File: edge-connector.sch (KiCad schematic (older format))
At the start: 3 parts

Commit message: Fixed libs
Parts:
- J?: footprint _autosave-artix-dc-scm-footprints:SFF-TA-1002-4C+ -> artix-dc-scm-footprints:SFF-TA-1002-4C+; symbol _autosave-artix-dc-scm:SFF-TA-1002-4C+ -> artix-dc-scm:SFF-TA-1002-4C+
- R136, R137: footprint _autosave-artix-dc-scm-footprints:0402-res -> artix-dc-scm-footprints:0402-res; symbol _autosave-artix-dc-scm:R_0R_0402 -> artix-dc-scm:R_0R_0402
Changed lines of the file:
@@
 Connection ~ 6925 10425
 $Comp
-L _autosave-artix-dc-scm:GND-artix-dc-scm #PWR026
+L artix-dc-scm:GND-artix-dc-scm #PWR026
 U 1 1 626F241B
 P 6925 10625
@@
 	8825 10425 8825 10625
 $Comp
-L _autosave-artix-dc-scm:GND-artix-dc-scm #PWR027
+L artix-dc-scm:GND-artix-dc-scm #PWR027
 U 1 1 62BB82B7
 P 8825 10625
@@
 $EndComp
 $Comp
-L _autosave-artix-dc-scm:R_0R_0402 R136
+L artix-dc-scm:R_0R_0402 R136
 U 1 1 616ABCDE
 P 9050 6725
 F 0 "R136" H 9050 6938 60  0000 C CNN
 F 1 "R_0R_0402" H 9050 6575 60  0001 C CNN
-F 2 "_autosave-artix-dc-scm-footprints:0402-res" H 9250 6925 60  0001 L CNN
+F 2 "artix-dc-scm-footprints:0402-res" H 9250 6925 60  0001 L CNN
 F 3 "" H 9050 6725 50  0001 C CNN
 F 4 "PANASONIC" H 9250 7125 60  0001 L CNN "Manufacturer"
@@
 SGPIO0_CLK
 $Comp
-L _autosave-artix-dc-scm:R_0R_0402 R137
+L artix-dc-scm:R_0R_0402 R137
 U 1 1 617019A6
 P 10275 6725
 F 0 "R137" H 10275 6938 60  0000 C CNN
 F 1 "R_0R_0402" H 10275 6575 60  0001 C CNN
-F 2 "_autosave-artix-dc-scm-footprints:0402-res" H 10475 6925 60  0001 L CNN
+F 2 "artix-dc-scm-footprints:0402-res" H 10475 6925 60  0001 L CNN
 F 3 "" H 10275 6725 50  0001 C CNN
 F 4 "PANASONIC" H 10475 7125 60  0001 L CNN "Manufacturer"
@@
 PCIE_HPM_TX[0]_P
 $Comp
-L _autosave-artix-dc-scm:SFF-TA-1002-4C+ J?
+L artix-dc-scm:SFF-TA-1002-4C+ J?
 U 1 1 601205AF
 P 7875 1425
 F 0 "J?" H 7875 1590 50  0000 C CNN
 F 1 "SFF-TA-1002-4C+" H 7875 1499 50  0000 C CNN
-F 2 "_autosave-artix-dc-scm-footprints:SFF-TA-1002-4C+" H 8025 1475 50  0001 C CNN
+F 2 "artix-dc-scm-footprints:SFF-TA-1002-4C+" H 8025 1475 50  0001 C CNN
 F 3 "https://cdn.amphenol-icc.com/media/wysiwyg/files/documentation/sme005.pdf?__cf_chl_jschl_tk__=4604d1306574a1ee474ea914090d3e0c57e266a6-1606907014-0-AbkYBTCTl__kMBcY3BDmgKpfUy32FqitwN2Lniuy8W-uyv2Ev04Q-Q5Mr7srIz_Wnur0_9chB4CRbxKSYcEh7IvAJYsUgJ0PWIS5YdRqqHg567uaZciEX2hQP4ss5l6M4XdNrxEjJppHvyRV3ku89t-VmUSzhgCb8oJlyHpTxST4dEmKZNXfM53TM0tmGirdVbCRt1Byrx5pkz_uMvNABIOj7B2-eDGK52J3DWRD76zEyjdxY7Iz11gPiOY5i_QGIR3uOwkR5LBPNXe8zGqAf8--AKa7RqDbIriQRt90_32C4zIuHqbGa05BXS135E65ov80PbVcb4eSiutCqcJUAacUwu3eVnXVeIumfihJxuP8Rv7_n6saeG_2IuQpEiskzovLGKZM3667Y-rm-AL1NRXTamtvBxqTk0vyMvZ60FgJ" H 8075 1375 50  0001 C CNN
 	1    7875 1425

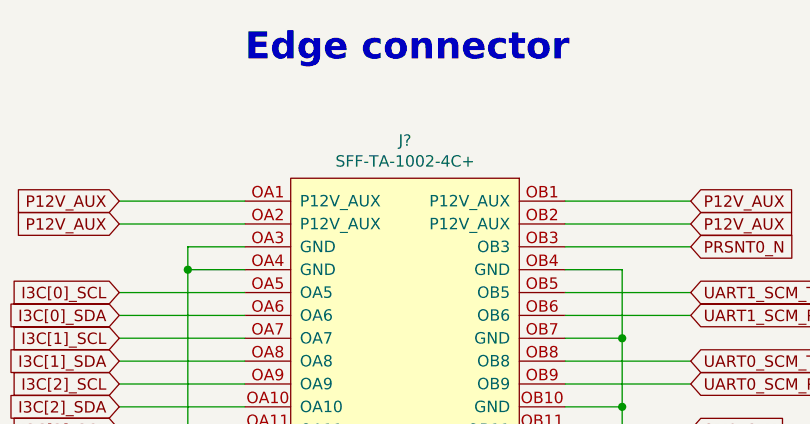
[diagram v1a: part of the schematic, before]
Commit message: update loclib
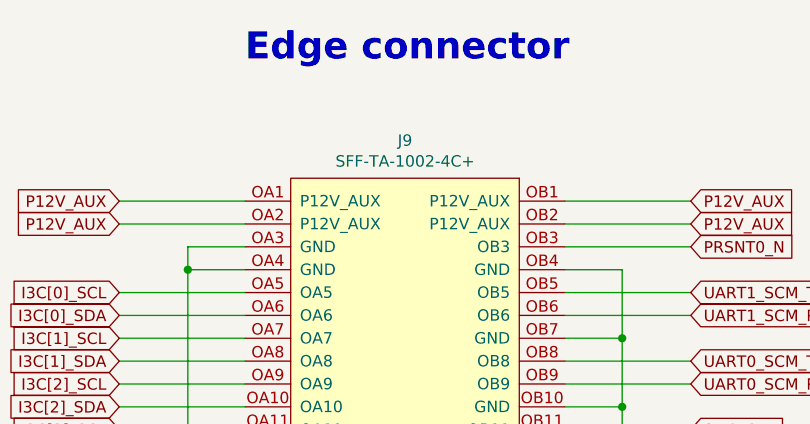
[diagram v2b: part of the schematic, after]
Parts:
- removed J?: SFF-TA-1002-4C+, artix-dc-scm-footprints:SFF-TA-1002-4C+, symbol artix-dc-scm:SFF-TA-1002-4C+
- added J9: SFF-TA-1002-4C+, artix-dc-scm-footprints:SFF-TA-1002-4C+, symbol artix-dc-scm:SFF-TA-1002-4C+
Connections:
- net 3V0_BAT: now also J9.B41
- net CHASI#: now also J9.A54
- net DBP_PRDY_N: now also J9.A50
- net DBP_PREQ_N: now also J9.A49
- net ESPI_ALERT_N: now also J9.B3
- net ESPI_CLK: now also J9.B1
- net ESPI_CS0_N: now also J9.B2
- net ESPI_CS1_N: now also J9.B9
- net ESPI_IO0: now also J9.B5
- net ESPI_IO1: now also J9.B6
- net ESPI_IO2: now also J9.B7
- net ESPI_IO3: now also J9.B8
- net ESPI_RESET_N: now also J9.B4
- net GND: now also J9.A11 (GND), J9.A14 (GND), J9.A17 (GND), J9.A20 (GND), J9.A33 (GND), J9.A42 (GND), J9.A58 (GND), J9.A61 (GND), J9.A64 (GND), J9.A67 (GND), J9.A70 (GND), J9.B10 (GND), J9.B17 (GND), J9.B26 (GND), J9.B33 (GND), J9.B38 (GND), J9.B49 (GND), J9.B52 (GND), J9.B55 (GND), J9.B58 (GND), J9.B61 (GND), J9.B64 (GND), J9.B67 (GND), J9.B70 (GND), J9.OA13 (GND), J9.OA3 (GND), J9.OA4 (GND), J9.OB10 (GND), J9.OB4 (GND), J9.OB7 (GND)
- net HPM_FW_RECOVERY: now also J9.A43
- net HPM_STBY_EN: now also J9.A45
- net HPM_STBY_RDY: now also J9.A44
- net HPM_STBY_RST_N: now also J9.A46
- net I2C[0]_SCL: now also J9.A1
- net I2C[0]_SDA: now also J9.A2
- net I2C[10]_SCL: now also J9.A31
- net I2C[10]_SDA: now also J9.A32
- net I2C[11]_SCL: now also J9.A38
- net I2C[11]_SDA: now also J9.A39
- net I2C[12]_SCL: now also J9.A40
- net I2C[12]_SDA: now also J9.A41
- net I2C[1]_SCL: now also J9.A3
- net I2C[1]_SDA: now also J9.A4
- net I2C[2]_SCL: now also J9.A5
- net I2C[2]_SDA: now also J9.A6
- net I2C[3]_SCL: now also J9.A7
- net I2C[3]_SDA: now also J9.A8
- net I2C[4]_SCL: now also J9.A9
- net I2C[4]_SDA: now also J9.A10
- net I2C[5]_SCL: now also J9.A21
- net I2C[5]_SDA: now also J9.A22
- net I2C[6]_SCL: now also J9.A23
- net I2C[6]_SDA: now also J9.A24
- net I2C[7]_SCL: now also J9.A25
- net I2C[7]_SDA: now also J9.A26
- net I2C[8]_SCL: now also J9.A27
- net I2C[8]_SDA: now also J9.A28
- net I2C[9]_SCL: now also J9.A29
- net I2C[9]_SDA: now also J9.A30
- net I3C[0]_SCL: now also J9.OA5
- net I3C[0]_SDA: now also J9.OA6
- net I3C[1]_SCL: now also J9.OA7
- net I3C[1]_SDA: now also J9.OA8
- net I3C[2]_SCL: now also J9.OA9
- net I3C[2]_SDA: now also J9.OA10
- net I3C[3]_SCL: now also J9.OA11
- net I3C[3]_SDA: now also J9.OA12
- net IRQ_N: now also J9.A56
- net JTAG_TCK: now also J9.A34
- net JTAG_TDI: now also J9.A36
- net JTAG_TDO: now also J9.A37
- net JTAG_TMS: now also J9.A35
- net NCSI_CLK: now also J9.B18
- net NCSI_CRS_DV: now also J9.B19
- net NCSI_RXD0: now also J9.B24
- net NCSI_RXD1: now also J9.B25
- net NCSI_RXER: now also J9.B23
- net NCSI_TXD0: now also J9.B21
- net NCSI_TXD1: now also J9.B22
- net NCSI_TXEN: now also J9.B20
- net P12V_AUX: now also J9.OA1 (P12V_AUX), J9.OA2 (P12V_AUX), J9.OB1 (P12V_AUX), J9.OB2 (P12V_AUX)
- net PCIE_BMC_CLK_100_N: now also J9.A13
- net PCIE_BMC_CLK_100_P: now also J9.A12
- net PCIE_BMC_RX_N: now also J9.A19
- net PCIE_BMC_RX_P: now also J9.A18
- net PCIE_BMC_TX_N: now also J9.A16
- net PCIE_BMC_TX_P: now also J9.A15
- net PCIE_HPM_CLK_N: now also J9.B57
- net PCIE_HPM_CLK_P: now also J9.B56
- net PCIE_HPM_RX[0]_N: now also J9.A60
- net PCIE_HPM_RX[0]_P: now also J9.A59
- net PCIE_HPM_RX[1]_N: now also J9.A63
- net PCIE_HPM_RX[1]_P: now also J9.A62
- net PCIE_HPM_RX[2]_N: now also J9.A66
- net PCIE_HPM_RX[2]_P: now also J9.A65
- net PCIE_HPM_RX[3]_N: now also J9.A69
- net PCIE_HPM_RX[3]_P: now also J9.A68
- net PCIE_HPM_TX[0]_N: now also J9.B60
- net PCIE_HPM_TX[0]_P: now also J9.B59
- net PCIE_HPM_TX[1]_N: now also J9.B63
- net PCIE_HPM_TX[1]_P: now also J9.B62
- net PCIE_HPM_TX[2]_N: now also J9.B66
- net PCIE_HPM_TX[2]_P: now also J9.B65
- net PCIE_HPM_TX[3]_N: now also J9.B69
- net PCIE_HPM_TX[3]_P: now also J9.B68
- net PECI_BMC: now also J9.B27
- net PRSNT0_N: now also J9.OB3
- net PRSNT1_N: now also J9.A57
- net PVCCIO_PECI: now also J9.B28
- net QSPI0_CLK: now also J9.B11
- net QSPI0_CS0_N: now also J9.B12
- net QSPI0_CS1_N: now also J9.B42
- net QSPI0_D0: now also J9.B13
- net QSPI0_D1: now also J9.B14
- net QSPI0_D2: now also J9.B15
- net QSPI0_D3: now also J9.B16
- net QSPI1_CLK: now also J9.B43
- net QSPI1_CS0_N: now also J9.B44
- net QSPI1_D0: now also J9.B45
- net QSPI1_D1: now also J9.B46
- net QSPI1_D2: now also J9.B47
- net QSPI1_D3: now also J9.B48
- net RST_PLTRST_BUF_N: now also J9.A51
- net RoT_CPU_RST_N: now also J9.A53
- net SGPIO0_CLK: now also J9.B30
- net SGPIO0_DI: now also J9.B31
- net SGPIO0_DO: now also J9.B29
- net SGPIO0_LD: now also J9.B32
- net SGPIO1_DI: now also J9.B36
- net SGPIO1_DO: now also J9.B34
- net SGPIO1_LD: now also J9.B37
- net SGPIO_INTR_N: now also J9.B40
- net SGPIO_RESET_N: now also J9.B39
- net SPARE0: now also J9.A55
- net SPARE1: now also J9.A52
- net SPI0_CLK: now also J9.OB11
- net SPI0_CS_N: now also J9.OB12
- net SPI0_MISO: now also J9.OB14
- net SPI0_MOSI: now also J9.OB13
- net SYS_PWRBTN_N: now also J9.A47
- net SYS_PWROK: now also J9.A48
- net UART0_SCM_RX: now also J9.OB9
- net UART0_SCM_TX: now also J9.OB8
- net UART1_SCM_RX: now also J9.OB6
- net UART1_SCM_TX: now also J9.OB5
- net USB1_D_N: now also J9.B54
- net USB1_D_P: now also J9.B53
- net USB2_D_N: now also J9.B51
- net USB2_D_P: now also J9.B50
- net VIRTUAL_RESEAT: now also J9.OA14
- net at R136.1: now also J9.B35
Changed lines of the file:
@@
 PCIE_HPM_TX[0]_P
 $Comp
-L artix-dc-scm:SFF-TA-1002-4C+ J?
-U 1 1 601205AF
+L artix-dc-scm:SFF-TA-1002-4C+ J9
+U 1 1 6012802C
 P 7875 1425
-F 0 "J?" H 7875 1590 50  0000 C CNN
+F 0 "J9" H 7875 1590 50  0000 C CNN
 F 1 "SFF-TA-1002-4C+" H 7875 1499 50  0000 C CNN
 F 2 "artix-dc-scm-footprints:SFF-TA-1002-4C+" H 8025 1475 50  0001 C CNN
